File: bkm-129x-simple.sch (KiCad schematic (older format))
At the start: 55 parts, among them J1 YG_IN, J11 YG_OUT, J2 PBB_IN, J21 PBB_OUT, J3 PRR_IN, J31 PRR_OUT, J4 SYNC_IN, J41 SYNC_OUT, J5 Conn_02x32_Row_Letter_Last, Q1 DTC144EKA, SW1 SW_YG_TERM, SW2 SW_PBB_TERM, SW3 SW_PRR_TERM, SW4 SW_SYNC_TERM, U1 ADG1611, U2 THS7374, U3 arduino-nano-v3, U4 74LVC125, U5 MIC3490-3.3

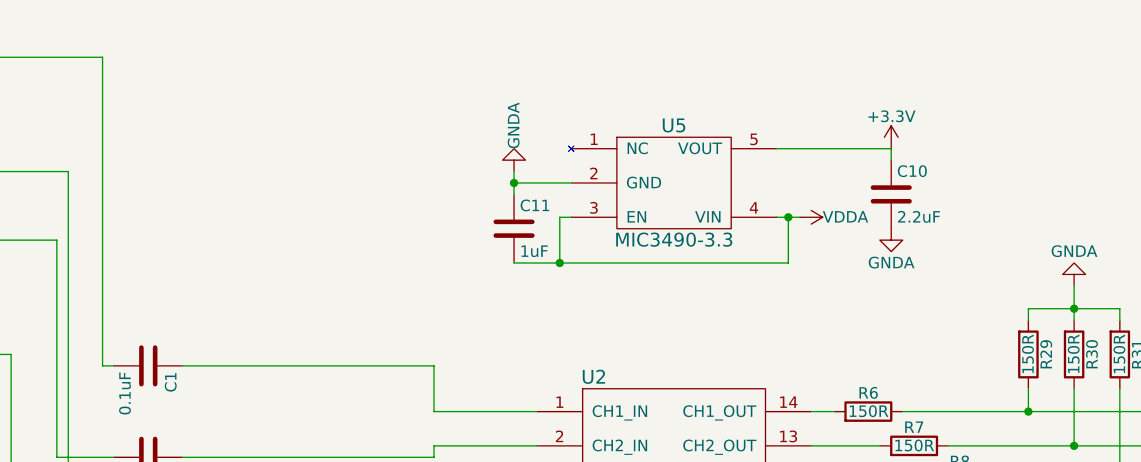
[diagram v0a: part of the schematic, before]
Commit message: Revision D
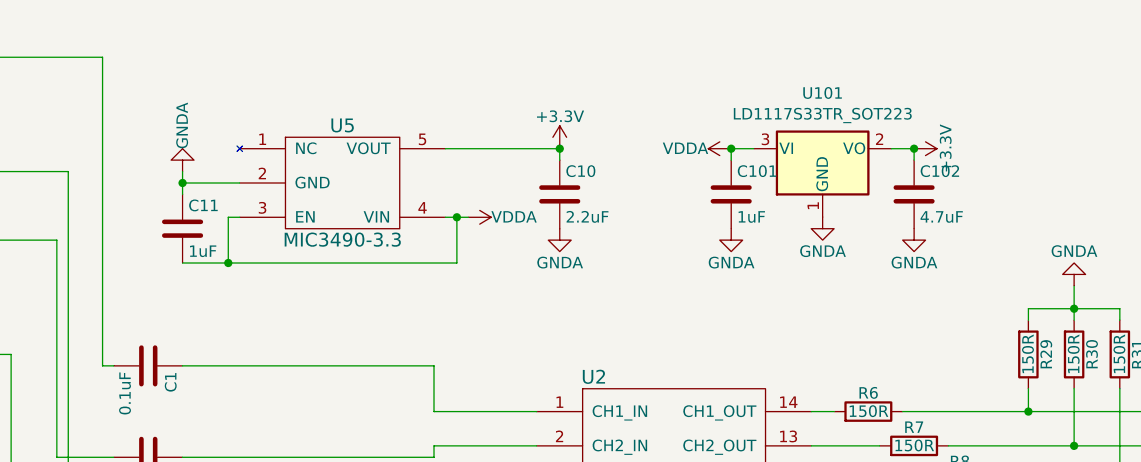
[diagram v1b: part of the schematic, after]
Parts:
- added C101: 1uF, Capacitor_SMD:C_0805_2012Metric_Pad1.18x1.45mm_HandSolder, symbol bkm-129x-simple-rescue:C
- added C102: 4.7uF, Capacitor_SMD:C_0805_2012Metric_Pad1.18x1.45mm_HandSolder, symbol bkm-129x-simple-rescue:C
- added U101: LD1117S33TR_SOT223, Package_TO_SOT_SMD:SOT-223-3_TabPin2, symbol Regulator_Linear:LD1117S33TR_SOT223
- C1, C10, C11, C12, C2, C3, C4, C5, C6, C9: footprint Capacitors_SMD:C_0805_HandSoldering -> Capacitor_SMD:C_0805_2012Metric_Pad1.18x1.45mm_HandSolder
- C13, C7, C8: footprint Capacitors_SMD:CP_Elec_6.3x5.3 -> Capacitor_SMD:CP_Elec_6.3x5.3
- J5: footprint din-41612-64p-ra:DIN-41612-64P -> standard-pin-64p-ra:STANDARD-PIN-64P-RA
- Q1: footprint TO_SOT_Packages_SMD:SC-59_Handsoldering -> Package_TO_SOT_SMD:SC-59_Handsoldering
- R1, R10, R11, R12, R13, R18, R19, R20, R21, R22, R23, R24, R25, R26, R27, R28, R29, R30, R31, R6, R7, R8, R9: footprint Resistors_SMD:R_0805_HandSoldering -> Resistor_SMD:R_0805_2012Metric_Pad1.20x1.40mm_HandSolder
- U1: footprint Housings_SSOP:TSSOP-16_4.4x5mm_Pitch0.65mm -> Package_SO:TSSOP-16_4.4x5mm_P0.65mm
- U2, U4: footprint Housings_SSOP:TSSOP-14_4.4x5mm_Pitch0.65mm -> Package_SO:TSSOP-14_4.4x5mm_P0.65mm
- U5: footprint TO_SOT_Packages_SMD:SOT-23-5_HandSoldering -> Package_TO_SOT_SMD:SOT-23-5_HandSoldering
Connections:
- net +3V3: now also C102.1, U101.2 (VO)
- net GND: now also C101.2, C102.2, U101.1 (GND)
- net VDD: now also C101.1, U101.3 (VI)
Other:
- moved on the sheet: C10, C11, U5
